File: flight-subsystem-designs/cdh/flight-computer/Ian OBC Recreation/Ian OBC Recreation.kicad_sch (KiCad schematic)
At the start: 42 parts, among them J8 Conn_02x26_Odd_Even, Q1 AON6411, Q2 AON6411, U1 BEAGLEBONEBLACK, U2 TPS2400DBVR, U3 TCAN337G, U4 MCP7940N-xSN, U5 ADM3485EARZ, U6 MAX706RESA+T, U7 TMP36xS, U8 TPS2400DBVR

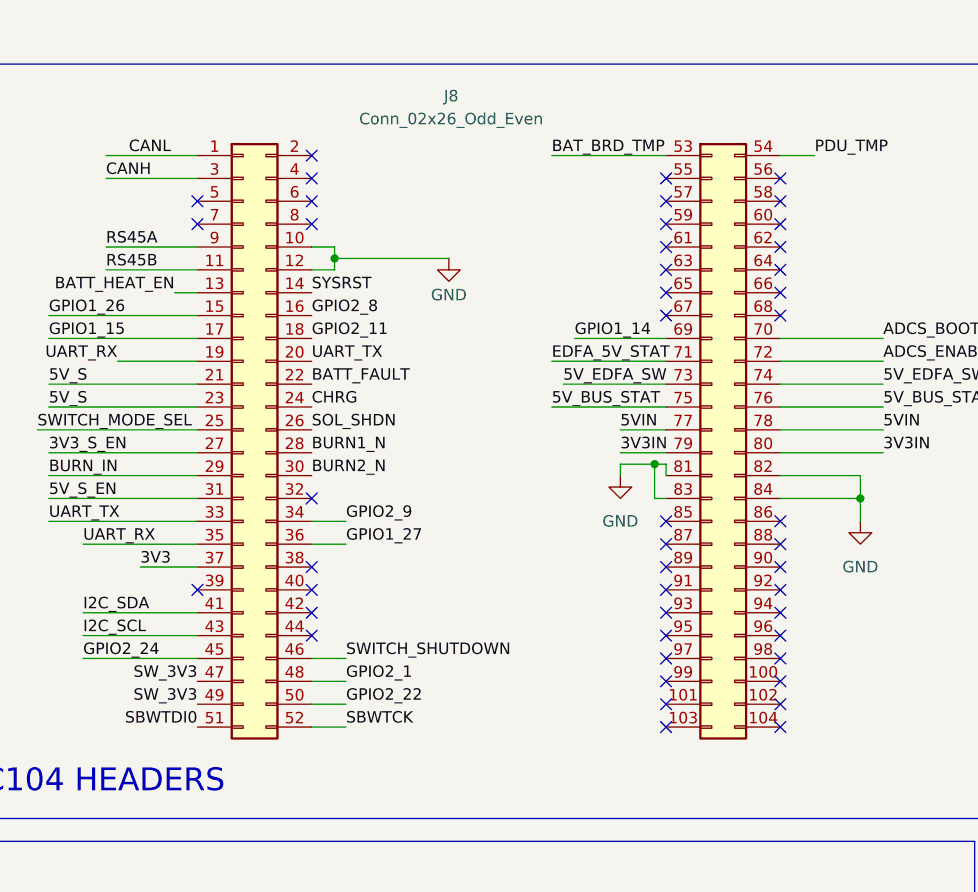
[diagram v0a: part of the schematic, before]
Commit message: Librecube Friendly Hopefully; Wiring Needs Work :C
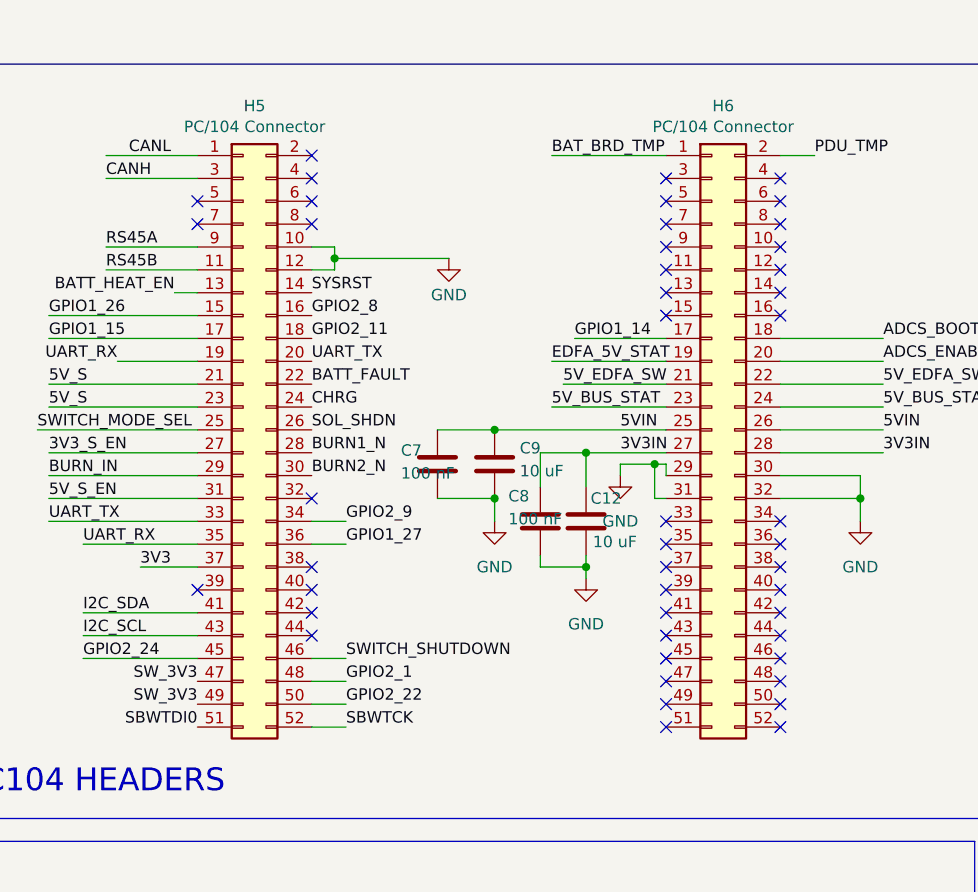
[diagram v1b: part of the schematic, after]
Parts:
- removed J8: Conn_02x26_Odd_Even, Footprints:LibreCube_PC104_4x26_P2.54mm_adjacent, symbol PC104:Conn_02x26_Odd_Even
- added C12, C9: 10 uF, symbol Device:C
- added C7, C8: 100 nF, symbol Device:C
- added H5, H6: PC/104 Connector, Connector_PinSocket_2.54mm:PinSocket_2x26_P2.54mm_Vertical, symbol Connector_Generic:Conn_02x26_Odd_Even
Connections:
- net 3V3IN: now also C12.1, C8.1, H6.27 (Pin_27), H6.28 (Pin_28)
- net 3V3_S_EN: now also H5.27 (Pin_27)
- net 5VIN: now also C7.1, C9.1, H6.25 (Pin_25), H6.26 (Pin_26)
- net 5V_BUS_STAT: now also H6.23 (Pin_23), H6.24 (Pin_24)
- net 5V_EDFA_SW: now also H6.21 (Pin_21), H6.22 (Pin_22)
- net 5V_S: now also H5.21 (Pin_21), H5.23 (Pin_23)
- net 5V_S_EN: now also H5.31 (Pin_31)
- net ADCS_BOOT: now also H6.18 (Pin_18)
- net ADCS_ENABLE: now also H6.20 (Pin_20)
- net BATT_FAULT: now also H5.22 (Pin_22)
- net BATT_HEAT_EN: now also H5.13 (Pin_13)
- net BAT_BRD_TMP: now also H6.1 (Pin_1)
- net BURN1_N: now also H5.28 (Pin_28)
- net BURN2_N: now also H5.30 (Pin_30)
- net BURN_IN: now also H5.29 (Pin_29)
- net CANH: now also H5.3 (Pin_3)
- net CANL: now also H5.1 (Pin_1)
- net CHRG: now also H5.24 (Pin_24)
- net DGND: now also C12.2, C7.2, C8.2, C9.2, H5.10 (Pin_10), H5.12 (Pin_12), H6.29 (Pin_29), H6.30 (Pin_30), H6.31 (Pin_31), H6.32 (Pin_32)
- net EDFA_5V_STAT: now also H6.19 (Pin_19)
- net GPIO1_14: now also H6.17 (Pin_17)
- net GPIO1_15: now also H5.17 (Pin_17)
- net GPIO1_26: now also H5.15 (Pin_15)
- net GPIO1_27: now also H5.36 (Pin_36)
- net GPIO2_1: now also H5.48 (Pin_48)
- net GPIO2_11: now also H5.18 (Pin_18)
- net GPIO2_22: now also H5.50 (Pin_50)
- net GPIO2_24: now also H5.45 (Pin_45)
- net GPIO2_8: now also H5.16 (Pin_16)
- net GPIO2_9: now also H5.34 (Pin_34)
- net I2C_SCL: now also H5.43 (Pin_43)
- net I2C_SDA: now also H5.41 (Pin_41)
- net PDU_TMP: now also H6.2 (Pin_2)
- net RS45A: now also H5.9 (Pin_9)
- net RS45B: now also H5.11 (Pin_11)
- net SBWTCK: now also H5.52 (Pin_52)
- net SBWTDI0: now also H5.51 (Pin_51)
- net SOL_SHDN: now also H5.26 (Pin_26)
- net SWITCH_MODE_SEL: now also H5.25 (Pin_25)
- net SWITCH_SHUTDOWN: now also H5.46 (Pin_46)
- net SW_3V3: now also H5.47 (Pin_47), H5.49 (Pin_49)
- net SYSRST: now also H5.14 (Pin_14)
- net UART_RX: now also H5.19 (Pin_19), H5.35 (Pin_35)
- net UART_TX: now also H5.20 (Pin_20), H5.33 (Pin_33)
- net VDD_3V3B: now also H5.37 (Pin_37)
